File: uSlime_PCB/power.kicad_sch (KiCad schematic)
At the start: 20 parts, among them CN2 1.25T-2AW, J1 USB_C_Receptacle_USB2.0_14P, U2 MSK-12C02_SMD_SPDT_SWITCH, U3 AP2112K-3.3TRG1, U4 MCP73831T-2ACI/OT

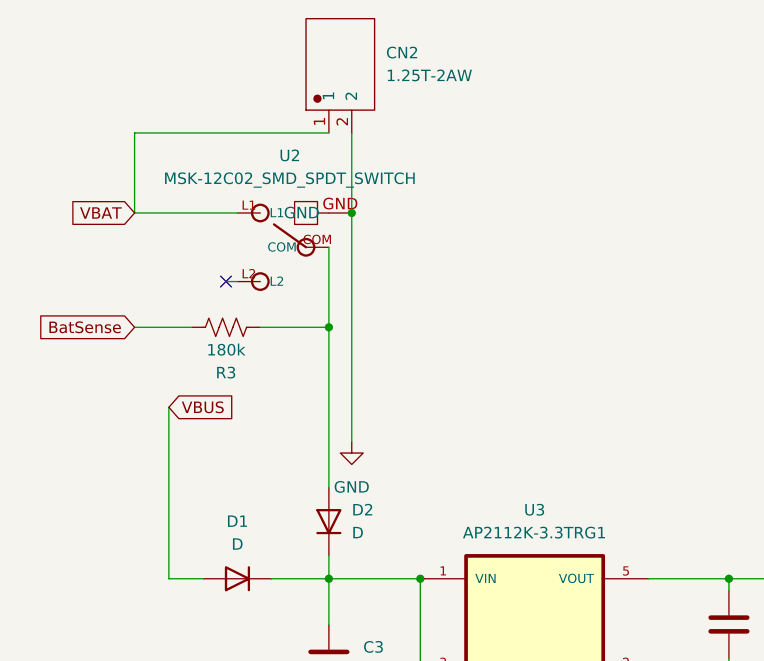
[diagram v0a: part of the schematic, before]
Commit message: Update main PCB schematic
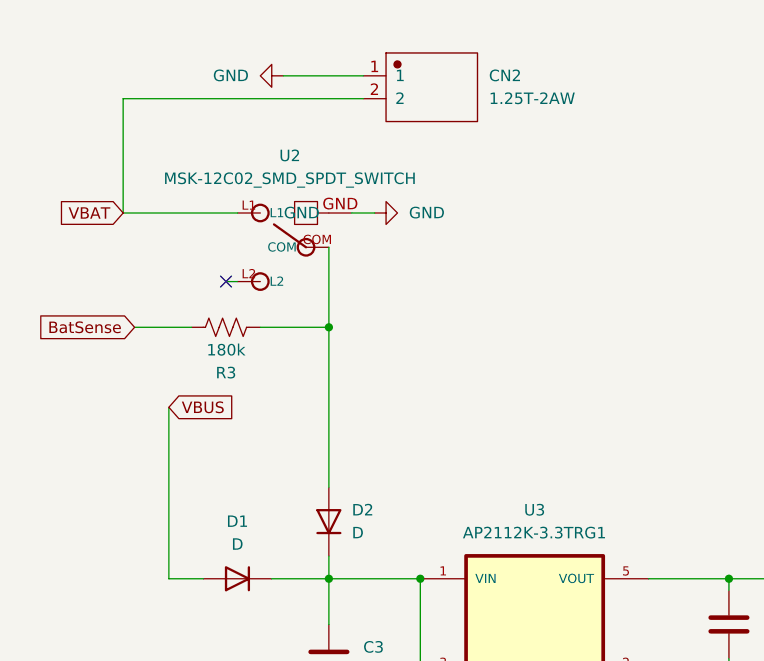
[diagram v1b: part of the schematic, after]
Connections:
- net GND: now also CN2.1; no longer CN2.2
- net VBAT: now also CN2.2; no longer CN2.1
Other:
- moved on the sheet: CN2
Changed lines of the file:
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@@
-	)
-	(junction
-		(at 69.85 36.83)
-		(diameter 0)
-		(color 0 0 0 0)
 	)
 	(junction
@@
 	(wire
 		(pts
-			(xy 67.31 27.94) (xy 45.72 27.94)
-		)
-		(stroke
-			(width 0)
-			(type default)
-		)
-	)
-	(wire
-		(pts
 			(xy 59.69 49.53) (xy 67.31 49.53)
 		)
@@
 	(wire
 		(pts
+			(xy 72.39 36.83) (xy 69.85 36.83)
+		)
+		(stroke
+			(width 0)
+			(type default)
+		)
+	)
+	(wire
+		(pts
 			(xy 163.83 135.89) (xy 166.37 135.89)
 		)
@@
 	(wire
 		(pts
+			(xy 62.23 21.59) (xy 71.12 21.59)
+		)
+		(stroke
+			(width 0)
+			(type default)
+		)
+	)
+	(wire
+		(pts
 			(xy 219.71 82.55) (xy 226.06 82.55)
 		)
@@
 	(wire
 		(pts
-			(xy 45.72 36.83) (xy 57.15 36.83)
+			(xy 44.45 36.83) (xy 57.15 36.83)
 		)
 		(stroke
@@
 		(pts
 			(xy 233.68 82.55) (xy 233.68 87.63)
-		)
-		(stroke
-			(width 0)
-			(type default)
-		)
-	)
-	(wire
-		(pts
-			(xy 69.85 27.94) (xy 69.85 36.83)
 		)
 		(stroke
@@
 	(wire
 		(pts
-			(xy 45.72 27.94) (xy 45.72 36.83)
+			(xy 44.45 24.13) (xy 44.45 36.83)
 		)
 		(stroke
@@
 	(wire
 		(pts
-			(xy 69.85 36.83) (xy 69.85 62.23)
-		)
-		(stroke
-			(width 0)
-			(type default)
-		)
-	)
-	(wire
-		(pts
 			(xy 140.97 156.21) (xy 148.59 156.21)
+		)
+		(stroke
+			(width 0)
+			(type default)
+		)
+	)
+	(wire
+		(pts
+			(xy 44.45 24.13) (xy 71.12 24.13)
 		)
 		(stroke
@@
 	(global_label "VBAT"
 		(shape input)
-		(at 45.72 36.83 180)
+		(at 44.45 36.83 180)
 		(fields_autoplaced yes)
 		(effects
@@
 		)
 		(property "Intersheetrefs" "${INTERSHEET_REFS}"
-			(at 38.32 36.83 0)
+			(at 37.05 36.83 0)
 			(effects
 				(font
@@
 	)
 	(symbol
+		(lib_id "power:GND")
+		(at 62.23 21.59 270)
+		(unit 1)
+		(exclude_from_sim no)
+		(in_bom yes)
+		(on_board yes)
+		(dnp no)
+		(fields_autoplaced yes)
+		(property "Reference" "#PWR017"
+			(at 55.88 21.59 0)
+			(effects
+				(font
+					(size 1.27 1.27)
+				)
+				(hide yes)
+			)
+		)
+		(property "Value" "GND"
+			(at 58.42 21.5899 90)
+			(effects
+				(font
+					(size 1.27 1.27)
+				)
+				(justify right)
+			)
+		)
+		(property "Footprint" ""
+			(at 62.23 21.59 0)
+			(effects
+				(font
+					(size 1.27 1.27)
+				)
+				(hide yes)
+			)
+		)
+		(property "Datasheet" ""
+			(at 62.23 21.59 0)
+			(effects
+				(font
+					(size 1.27 1.27)
+				)
+				(hide yes)
+			)
+		)
+		(property "Description" "Power symbol creates a global label with name \"GND\" , ground"
+			(at 62.23 21.59 0)
+			(effects
+				(font
+					(size 1.27 1.27)
+				)
+				(hide yes)
+			)
+		)
+		(pin "1"
+		)
+		(instances
+			(project "uSlime"
+				(path "/f32c1c49-f803-4e7c-a530-6db148a7ba36/9141278c-15a6-43aa-8c9d-f1bdf7efadba"
+					(reference "#PWR017")
+					(unit 1)
+				)
+			)
+		)
+	)
+	(symbol
 		(lib_id "uSlime:D")
 		(at 67.31 71.12 90)
@@
 	(symbol
 		(lib_id "uSlime:1.25T-2AW")
-		(at 68.58 21.59 90)
+		(at 77.47 22.86 0)
 		(unit 1)
 		(exclude_from_sim no)
@@
 		(fields_autoplaced yes)
 		(property "Reference" "CN2"
-			(at 73.66 19.0499 90)
-			(effects
-				(font
-					(size 1.27 1.27)
-				)
-				(justify right)
+			(at 85.09 21.5899 0)
+			(effects
+				(font
+					(size 1.27 1.27)
+				)
+				(justify left)
 			)
 		)
 		(property "Value" "1.25T-2AW"
-			(at 73.66 21.5899 90)
-			(effects
-				(font
-					(size 1.27 1.27)
-				)
-				(justify right)
+			(at 85.09 24.1299 0)
+			(effects
+				(font
+					(size 1.27 1.27)
+				)
+				(justify left)
 			)
 		)
 		(property "Footprint" "uSlime-libs:CONN-TH_2P-P1.25_1.25T-2AW"
-			(at 67.1576 21.59 0)
+			(at 77.47 21.4376 0)
 			(effects
 				(font
@@
 		)
 		(property "Datasheet" "http://www.szlcsc.com/product/details_157311.html"
-			(at 72.2376 21.59 0)
+			(at 77.47 26.5176 0)
 			(effects
 				(font
@@
 		)
 		(property "Description" "C145979"
-			(at 77.3176 21.59 0)
+			(at 77.47 31.5976 0)
 			(effects
 				(font
@@
 		)
 		(property "uuid" "std:acc09904c2b24521a5e7f02a7fa98dec"
-			(at 77.3176 21.59 0)
+			(at 77.47 31.5976 0)
 			(effects
 				(font
@@
 	(symbol
 		(lib_id "power:GND")
-		(at 69.85 62.23 0)
+		(at 72.39 36.83 90)
 		(unit 1)
 		(exclude_from_sim no)
@@
 		(fields_autoplaced yes)
 		(property "Reference" "#PWR03"
-			(at 69.85 68.58 0)
+			(at 78.74 36.83 0)
 			(effects
 				(font
@@
 		)
 		(property "Value" "GND"
-			(at 69.85 67.31 0)
-			(effects
-				(font
-					(size 1.27 1.27)
-				)
+			(at 76.2 36.8299 90)
+			(effects
+				(font
+					(size 1.27 1.27)
+				)
+				(justify right)
 			)
 		)
 		(property "Footprint" ""
-			(at 69.85 62.23 0)
+			(at 72.39 36.83 0)
 			(effects
 				(font
@@
 		)
 		(property "Datasheet" ""
-			(at 69.85 62.23 0)
+			(at 72.39 36.83 0)
 			(effects
 				(font
@@
 		)
 		(property "Description" "Power symbol creates a global label with name \"GND\" , ground"
-			(at 69.85 62.23 0)
-			(effects
-				(font
+			(at 72.39 36.83 0)
+			(effects
+				(font
